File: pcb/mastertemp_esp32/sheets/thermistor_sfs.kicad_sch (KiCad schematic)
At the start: 21 parts, among them J4 THERMISTOR_2P, U14 THERMISTOR_AFE_TBD, U16 THERM_WINDOW_TLV6700_TBD, U17 SFS_WINDOW_TLV6700_TBD, U18 SFS_AFE_BUFFER_TBD, U7 ADS1115IDGSR_CANDIDATE

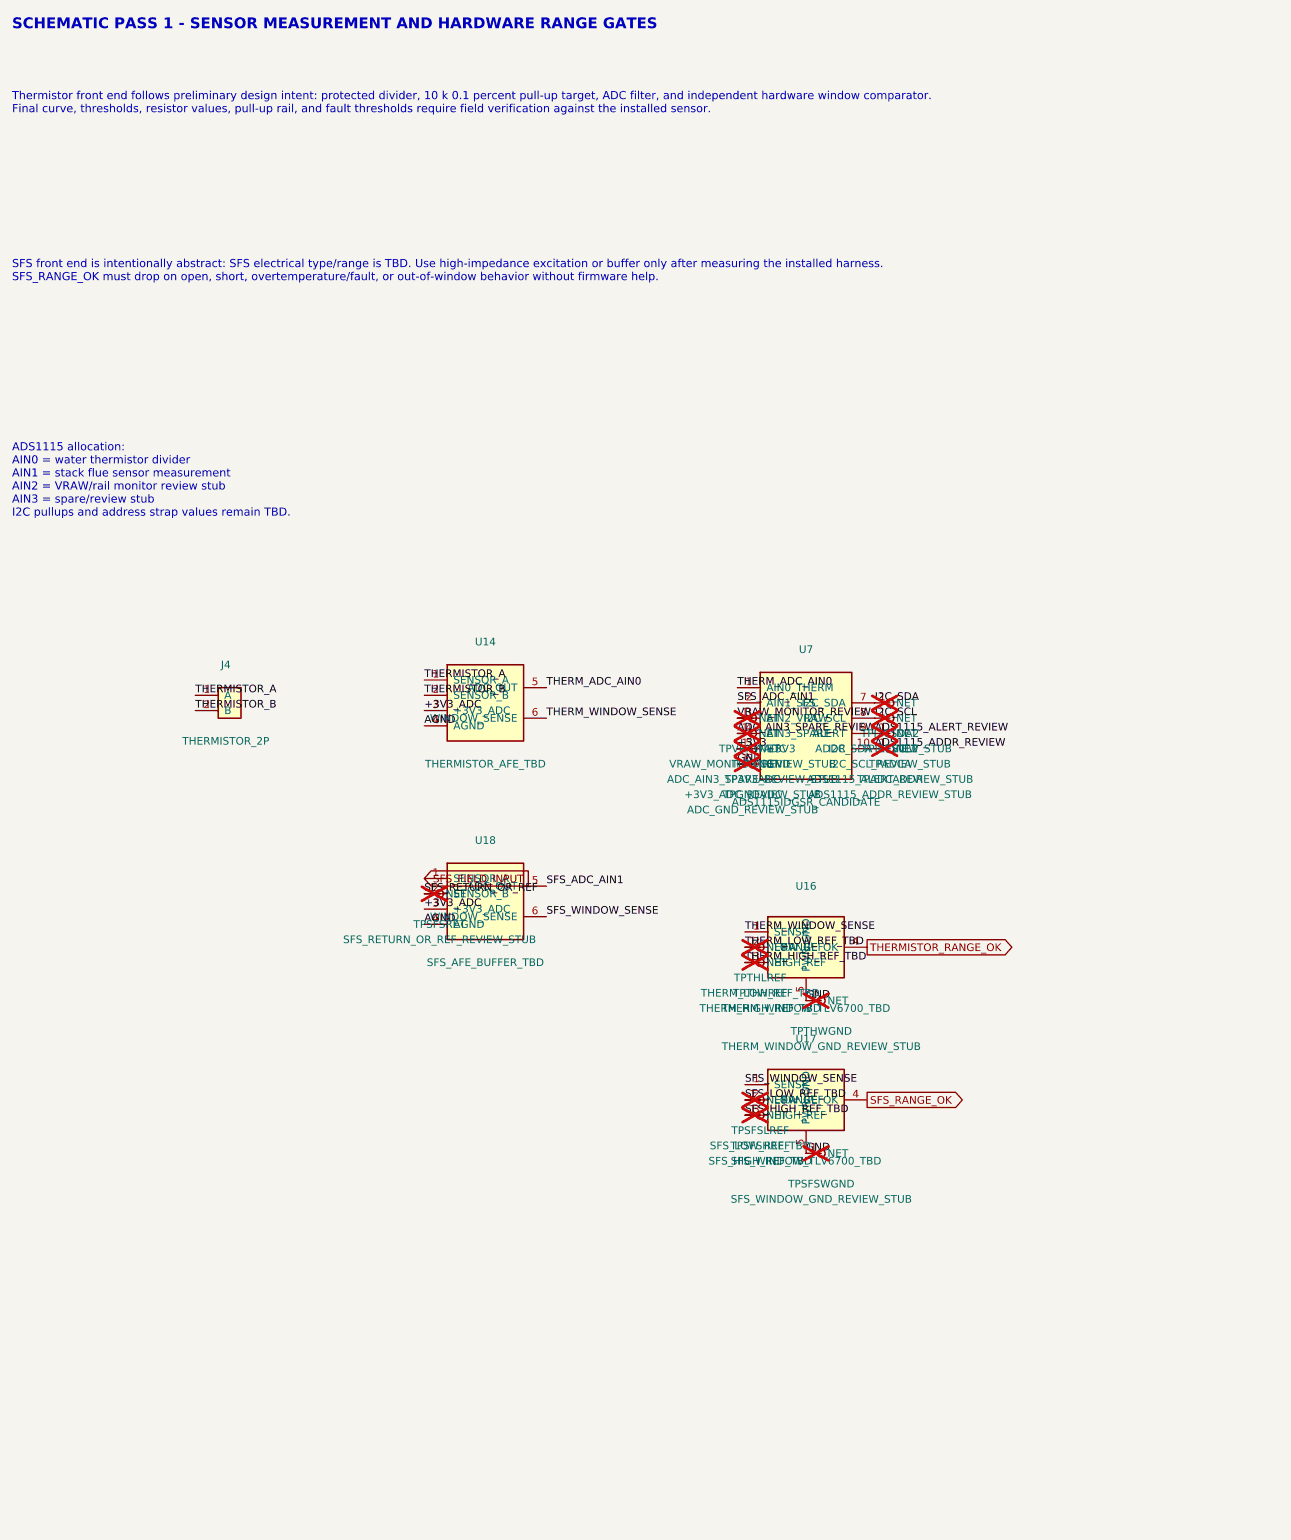
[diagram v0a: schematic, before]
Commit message: AI
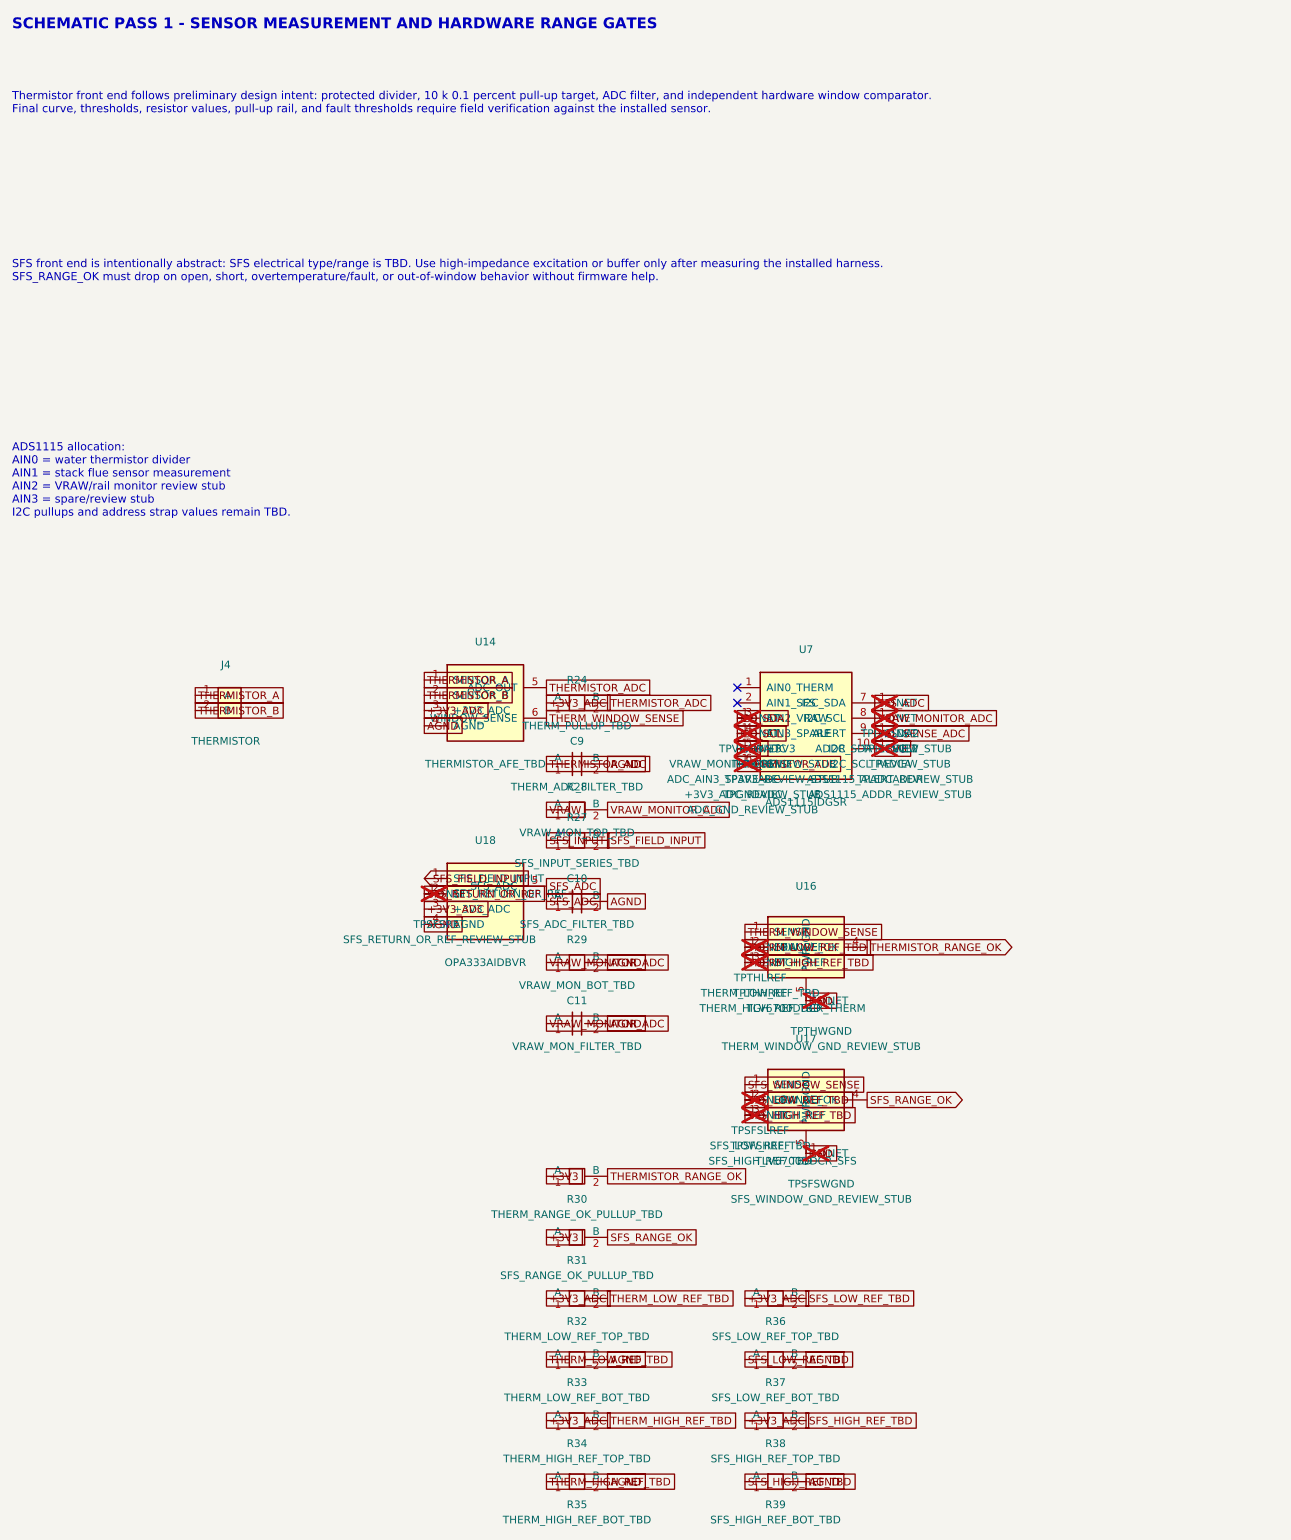
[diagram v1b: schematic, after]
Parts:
- added C10: SFS_ADC_FILTER_TBD, Capacitor_SMD:C_0805_2012Metric, symbol mastertemp_esp32:Capacitor_2pin
- added C11: VRAW_MON_FILTER_TBD, Capacitor_SMD:C_0805_2012Metric, symbol mastertemp_esp32:Capacitor_2pin
- added C9: THERM_ADC_FILTER_TBD, Capacitor_SMD:C_0805_2012Metric, symbol mastertemp_esp32:Capacitor_2pin
- added R24: THERM_PULLUP_TBD, Resistor_SMD:R_0805_2012Metric, symbol mastertemp_esp32:Resistor_2pin
- added R27: SFS_INPUT_SERIES_TBD, Resistor_SMD:R_0805_2012Metric, symbol mastertemp_esp32:Resistor_2pin
- added R28: VRAW_MON_TOP_TBD, Resistor_SMD:R_0805_2012Metric, symbol mastertemp_esp32:Resistor_2pin
- added R29: VRAW_MON_BOT_TBD, Resistor_SMD:R_0805_2012Metric, symbol mastertemp_esp32:Resistor_2pin
- added R30: THERM_RANGE_OK_PULLUP_TBD, Resistor_SMD:R_0805_2012Metric, symbol mastertemp_esp32:Resistor_2pin
- added R31: SFS_RANGE_OK_PULLUP_TBD, Resistor_SMD:R_0805_2012Metric, symbol mastertemp_esp32:Resistor_2pin
- added R32: THERM_LOW_REF_TOP_TBD, Resistor_SMD:R_0805_2012Metric, symbol mastertemp_esp32:Resistor_2pin
- added R33: THERM_LOW_REF_BOT_TBD, Resistor_SMD:R_0805_2012Metric, symbol mastertemp_esp32:Resistor_2pin
- added R34: THERM_HIGH_REF_TOP_TBD, Resistor_SMD:R_0805_2012Metric, symbol mastertemp_esp32:Resistor_2pin
- added R35: THERM_HIGH_REF_BOT_TBD, Resistor_SMD:R_0805_2012Metric, symbol mastertemp_esp32:Resistor_2pin
- added R36: SFS_LOW_REF_TOP_TBD, Resistor_SMD:R_0805_2012Metric, symbol mastertemp_esp32:Resistor_2pin
- added R37: SFS_LOW_REF_BOT_TBD, Resistor_SMD:R_0805_2012Metric, symbol mastertemp_esp32:Resistor_2pin
- added R38: SFS_HIGH_REF_TOP_TBD, Resistor_SMD:R_0805_2012Metric, symbol mastertemp_esp32:Resistor_2pin
- added R39: SFS_HIGH_REF_BOT_TBD, Resistor_SMD:R_0805_2012Metric, symbol mastertemp_esp32:Resistor_2pin
- J4: value THERMISTOR_2P -> THERMISTOR; footprint TerminalBlock_Phoenix:PhoenixContact_MSTBA_2,5_2-G-5,08_1x02_P5.08mm_Horizontal -> Connector_Phoenix_MSTB:PhoenixContact_MSTBA_2,5_2-G-5,08_1x02_P5.08mm_Horizontal
- U14: footprint (none) -> Package_TO_SOT_SMD:SOT-23-6
- U16: value THERM_WINDOW_TLV6700_TBD -> TLV6700DDCR_THERM
- U17: value SFS_WINDOW_TLV6700_TBD -> TLV6700DDCR_SFS
- U18: value SFS_AFE_BUFFER_TBD -> OPA333AIDBVR; symbol mastertemp_esp32:SensorAFE_6pin -> mastertemp_esp32:SFSBuffer_5pin
- U7: value ADS1115IDGSR_CANDIDATE -> ADS1115IDGSR
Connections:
- net ADC_AIN3_SPARE_REVIEW is gone; now on net I2C_SCL: TPADC3.1 (NET), U7.4 (AIN3_SPARE)
- net ADS1115_ADDR_REVIEW is gone; now on net +3V3: TPADCADDR.1 (NET), U7.10 (ADDR)
- net VRAW_MONITOR_REVIEW is gone; now on net I2C_SDA: TPVRAWADC.1 (NET), U7.3 (AIN2_VRAW)
- net +3V3: now also R30.1 (A), R31.1 (A); no longer TP3V3ADC.1 (NET), U7.5 (+3V3)
- net +3V3_ADC: now also R24.1 (A), R32.1 (A), R34.1 (A), R36.1 (A), R38.1 (A)
- net AGND: now also C10.2 (B), C11.2 (B), C9.2 (B), R29.2 (B), R33.2 (B), R35.2 (B), R37.2 (B), R39.2 (B)
- net GND: now also TP3V3ADC.1 (NET), U7.5 (+3V3); no longer TPGNDADC.1 (NET), U7.6 (GND)
- net I2C_SCL: no longer TPI2CSCL2.1 (NET), U7.8 (I2C_SCL)
- net I2C_SDA: no longer TPI2CSDA2.1 (NET), U7.7 (I2C_SDA)
- net SFS_FIELD_INPUT: now also R27.2 (B)
- net SFS_HIGH_REF_TBD: now also R38.2 (B), R39.1 (A)
- net SFS_LOW_REF_TBD: now also R36.2 (B), R37.1 (A)
- net SFS_RANGE_OK: now also R31.2 (B)
- net SFS_WINDOW_SENSE: no longer U18.6 (WINDOW_SENSE)
- net THERMISTOR_RANGE_OK: now also R30.2 (B)
- net THERM_HIGH_REF_TBD: now also R34.2 (B), R35.1 (A)
- net THERM_LOW_REF_TBD: now also R32.2 (B), R33.1 (A)
- net ADS1115_ALERT_REVIEW renamed VAL_SENSE_ADC
- net SFS_ADC_AIN1: no longer names the net of U7.2 (AIN1_SFS)
- net SFS_ADC_AIN1: no longer U18.5 (ADC_OUT)
- net THERM_ADC_AIN0: no longer names the net of U7.1 (AIN0_THERM)
- net THERM_ADC_AIN0: no longer U14.5 (ADC_OUT)
- new net SFS_ADC: C10.1 (A), TPI2CSDA2.1 (NET), U18.5 (SFS_ADC), U7.7 (I2C_SDA)
- new net SFS_INPUT: R27.1 (A)
- new net THERMISTOR_ADC: C9.1 (A), R24.2 (B), TPGNDADC.1 (NET), U14.5 (ADC_OUT), U7.6 (GND)
- new net VRAW: R28.1 (A)
- new net VRAW_MONITOR_ADC: C11.1 (A), R28.2 (B), R29.1 (A), TPI2CSCL2.1 (NET), U7.8 (I2C_SCL)
- no-connect marks 0 -> 2
